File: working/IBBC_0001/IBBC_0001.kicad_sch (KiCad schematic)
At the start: 11 parts, among them J1 HEAD-I01-X-PI10-01 oom.lt/H10, J2 HEAD-I01-X-PI04-01 oom.lt/H4, J3 HEAD-JSTSH-X-PI04-RS oom.lt/H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, J4 HEAD-JSTSH-X-PI04-RS oom.lt/H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, U1 AP2112K-3.3, U2 ADXL343

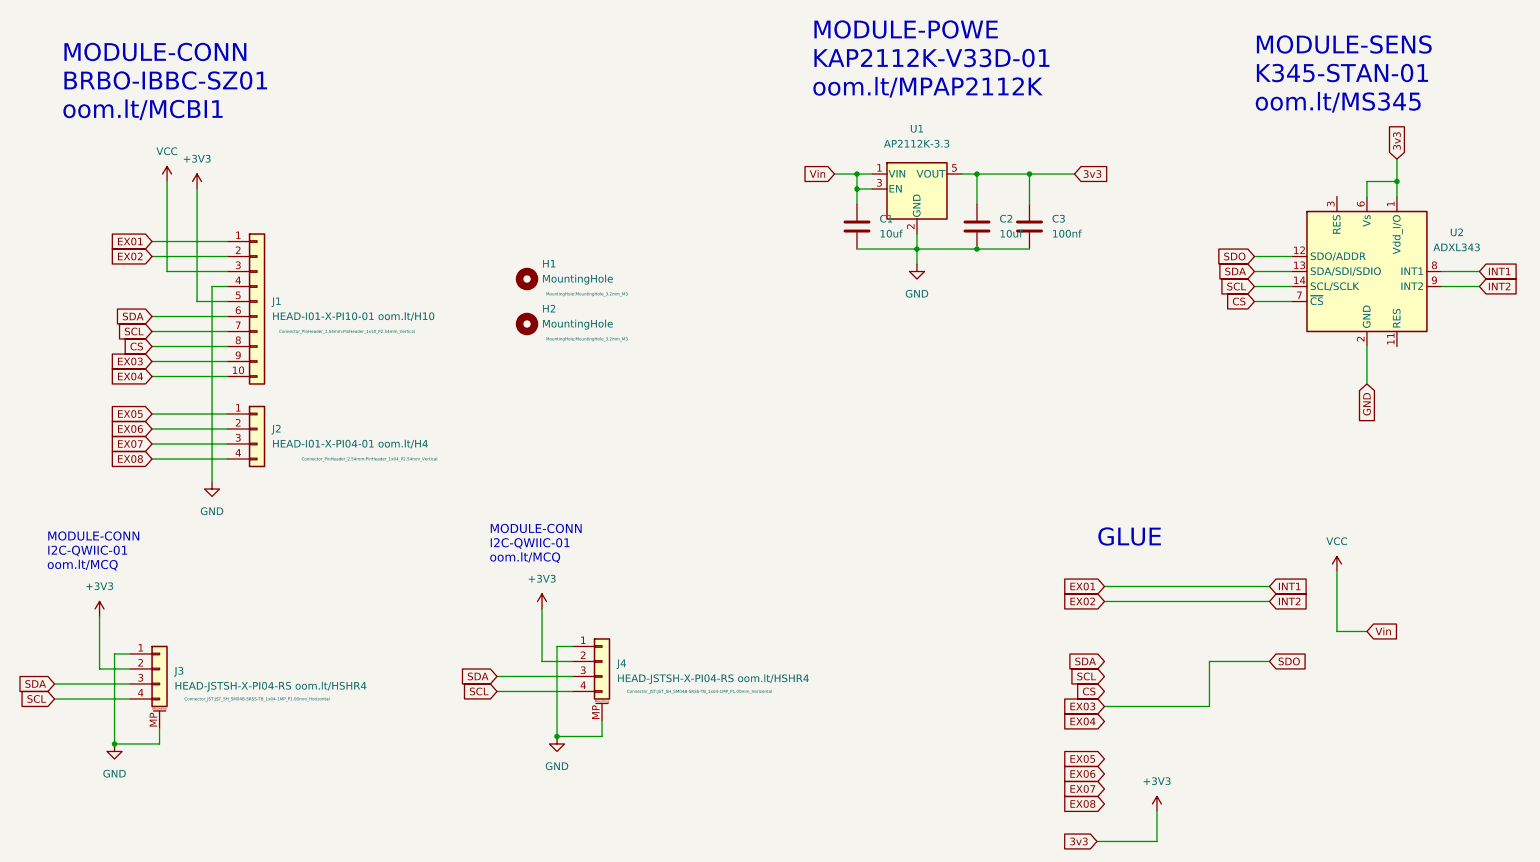
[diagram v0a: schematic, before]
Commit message: Workings.
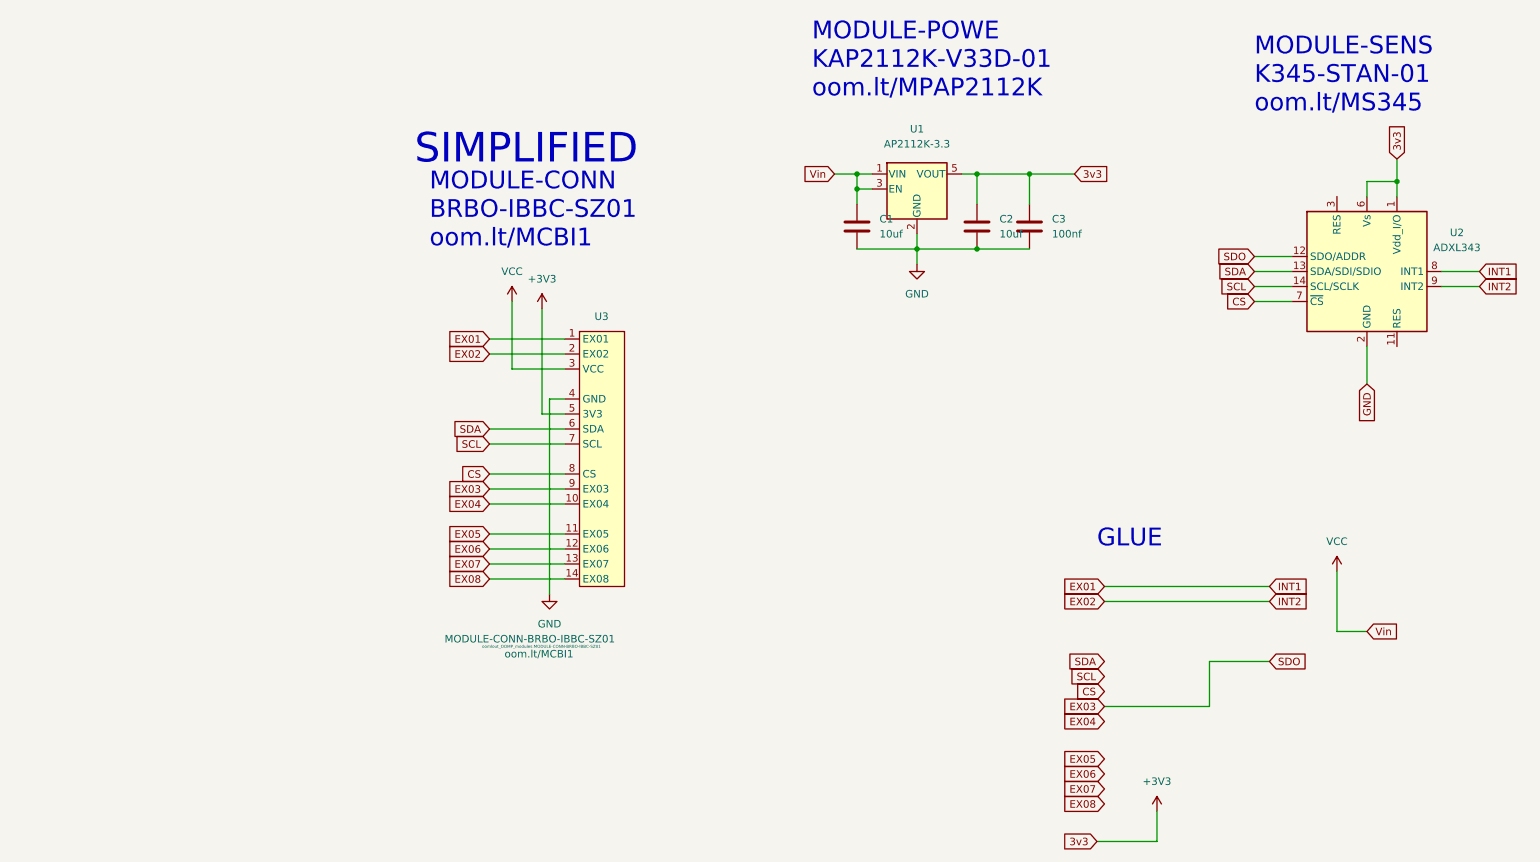
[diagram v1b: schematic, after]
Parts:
- removed H1, H2: MountingHole, MountingHole:MountingHole_3.2mm_M3, symbol Mechanical:MountingHole
- removed J1: HEAD-I01-X-PI10-01 oom.lt/H10, Connector_PinHeader_2.54mm:PinHeader_1x10_P2.54mm_Vertical, symbol Connector_Generic:Conn_01x10
- removed J2: HEAD-I01-X-PI04-01 oom.lt/H4, Connector_PinHeader_2.54mm:PinHeader_1x04_P2.54mm_Vertical, symbol Connector_Generic:Conn_01x04
- removed J3, J4: HEAD-JSTSH-X-PI04-RS oom.lt/HSHR4, Connector_JST:JST_SH_SM04B-SRSS-TB_1x04-1MP_P1.00mm_Horizontal, symbol Connector_Generic_MountingPin:Conn_01x04_MountingPin
- added U3: MODULE-CONN-BRBO-IBBC-SZ01, oomlout_OOMP_modules:MODULE-CONN-BRBO-IBBC-SZ01, symbol oomlout_OOMP_modules:MODULE-CONN-BRBO-IBBC-SZ01
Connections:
- net +3V3: now also U3.5 (3V3)
- net CS: now also U3.8 (CS)
- net EX01: now also U3.1 (EX01)
- net EX02: now also U3.2 (EX02)
- net EX03: now also U3.9 (EX03)
- net EX04: now also U3.10 (EX04)
- net EX05: now also U3.11 (EX05)
- net EX06: now also U3.12 (EX06)
- net EX07: now also U3.13 (EX07)
- net EX08: now also U3.14 (EX08)
- net GND: now also U3.4 (GND)
- net SCL: now also U3.7 (SCL)
- net SDA: now also U3.6 (SDA)
- net VCC: now also U3.3 (VCC)
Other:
- note added: "SIMPLIFIED"
- note removed: "MODULE-CONN I2C-QWIIC-01 oom.lt/MCQ"
